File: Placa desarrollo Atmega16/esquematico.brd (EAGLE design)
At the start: 93.7 x 90.2 mm, 34 parts, among them IC1 MEGA16-P, IC2 7805DT, IC3 7805DT, Q2 16MHz, X1 PN61729-S

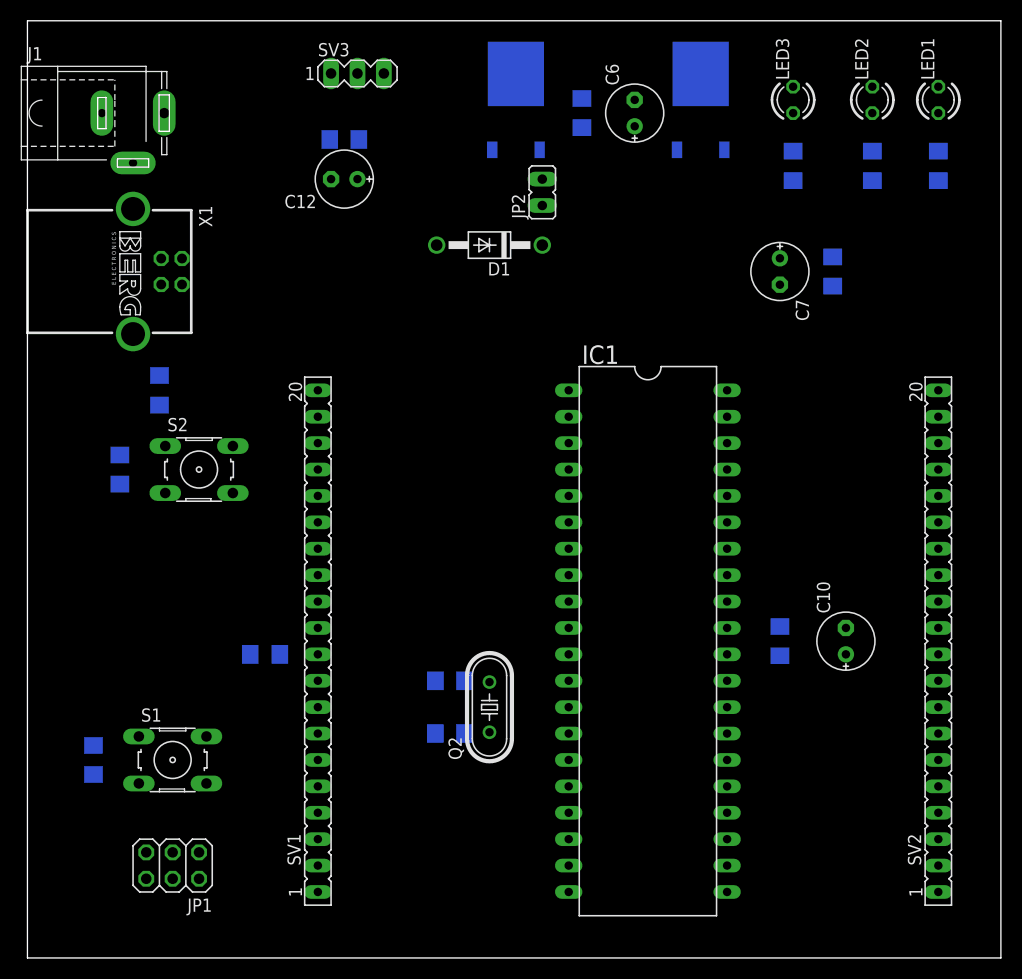
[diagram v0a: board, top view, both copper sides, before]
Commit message: PCB ruteado
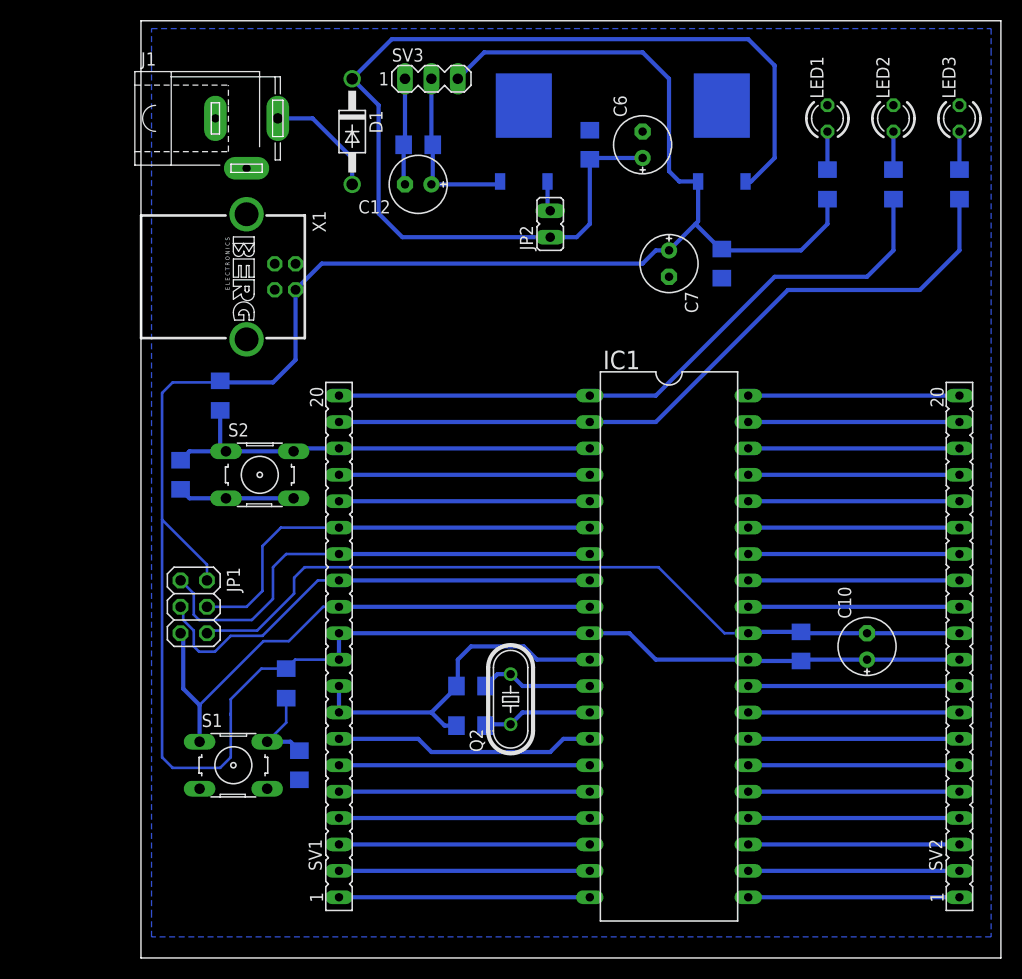
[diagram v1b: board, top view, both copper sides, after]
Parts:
- moved JP1 25.0 mm to (22.4, 33.8), turned to 270 degrees
- moved C1 19.8 mm to (32.5, 18.5)
- moved D1 17.1 mm to (37.6, 79.5), turned to 270 degrees
- moved LED3 16.1 mm to (96.0, 80.8)
- moved R4 16.1 mm to (96.0, 74.4)
- moved X1 10.9 mm to (27.4, 65.5)
- moved J1 10.9 mm to (27.4, 80.8)
- moved R2 10.8 mm to (83.3, 74.4)
- moved LED1 10.8 mm to (83.3, 80.8)
- moved C5 10.7 mm to (73.2, 66.8)
- moved C7 10.7 mm to (68.1, 66.8)
- moved C11 7.13 mm to (43.9, 78.2)
- moved C12 7.13 mm to (43.9, 74.4)
- moved SV3 7.13 mm to (45.2, 84.6)
- moved S2 5.86 mm to (28.7, 46.5)
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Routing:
- net VCC_5V: track 0.00 -> 249.1 mm
- net GND: track 0.00 -> 134.4 mm
- net VIN: track 0.00 -> 103.0 mm
- net PB1: track 0.00 -> 71.5 mm
- net PB0: track 0.00 -> 64.1 mm
- net RESET: track 0.00 -> 61.1 mm
- net MISO: track 0.00 -> 46.6 mm
- net SCK: track 0.00 -> 46.5 mm
- net PB2: track 0.00 -> 43.8 mm
- net MOSI: track 0.00 -> 42.5 mm
- net PD0: track 0.00 -> 25.2 mm
- net PD6: track 0.00 -> 24.1 mm
- net PD5: track 0.00 -> 24.1 mm
- net PD4: track 0.00 -> 24.1 mm
- net PD3: track 0.00 -> 24.1 mm
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- added copper zone on layer 16, net GND
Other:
- board size 93.7 x 90.2 mm -> 82.7 x 90.2 mm
